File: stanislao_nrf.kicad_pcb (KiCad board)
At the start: 2 copper layers, 53.5 x 21 mm, 19 parts, among them J1 Conn_01x06, Q1 BTS4140N, Q2 BSP89, U1 NRF52840-DONGLE, U2 LM5007MM

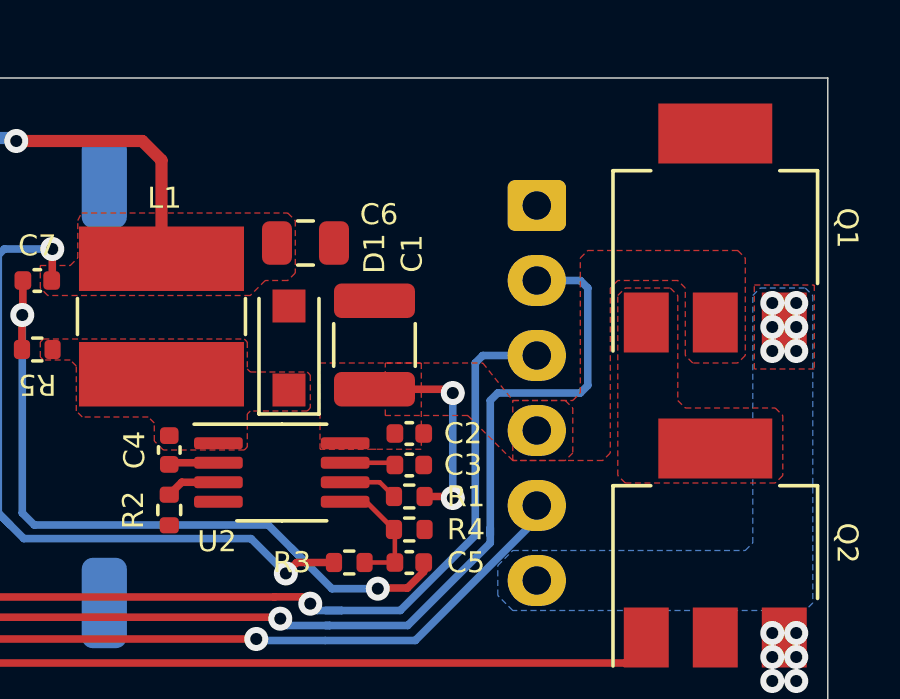
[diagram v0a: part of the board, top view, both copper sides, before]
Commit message: Non chinese version
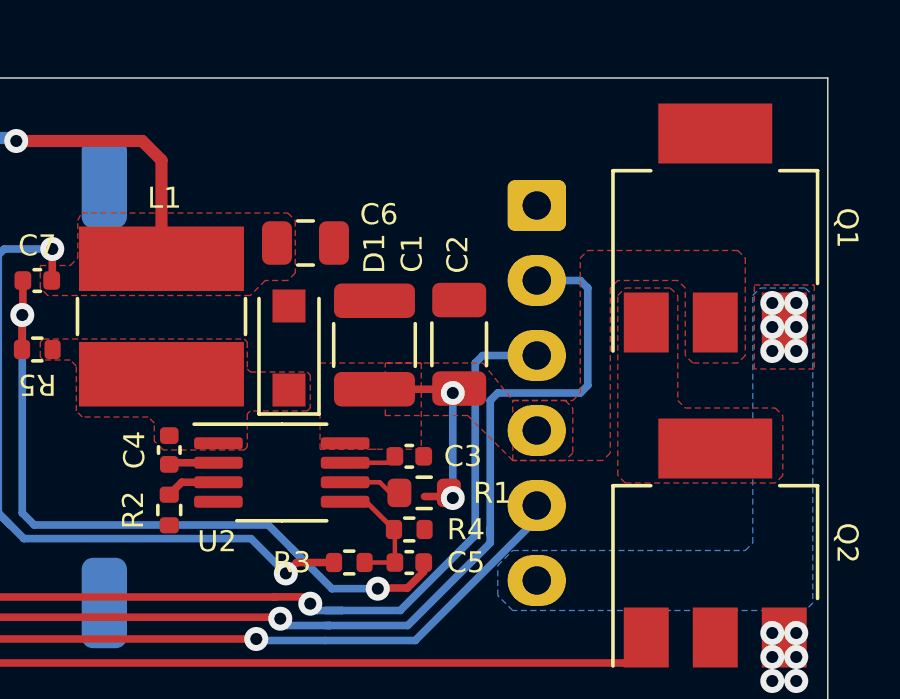
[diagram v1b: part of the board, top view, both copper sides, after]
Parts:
- C2: footprint Capacitor_SMD:C_0402_1005Metric -> Capacitor_SMD:C_1206_3216Metric
- R1: footprint Resistor_SMD:R_0402_1005Metric -> Resistor_SMD:R_0603_1608Metric
- moved C2 3.41 mm to (93.0, 68.4), turned to 90 degrees
- moved R1 0.51 mm to (91.8, 73.3)
- moved C3 0.29 mm to (91.3, 72.1)
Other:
- board text added: "BRAKE"
- board text added: "GND"
- board text added: "RX"
- board text added: "TX"
- board text added: "VIN"
- board text added: "V_BATT"
